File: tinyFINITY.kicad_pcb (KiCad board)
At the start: 2 copper layers, 20 x 20 mm, 111 parts, among them U1 MIC5205, U2 RTC6705, U3 ts3a44159, U4 STM32F301K8Ux, U5 TPS62153A-Q1, X1 8MHZ 20pF 30ppm, X2 8MHz, Y1 LF2012-A5R5AA

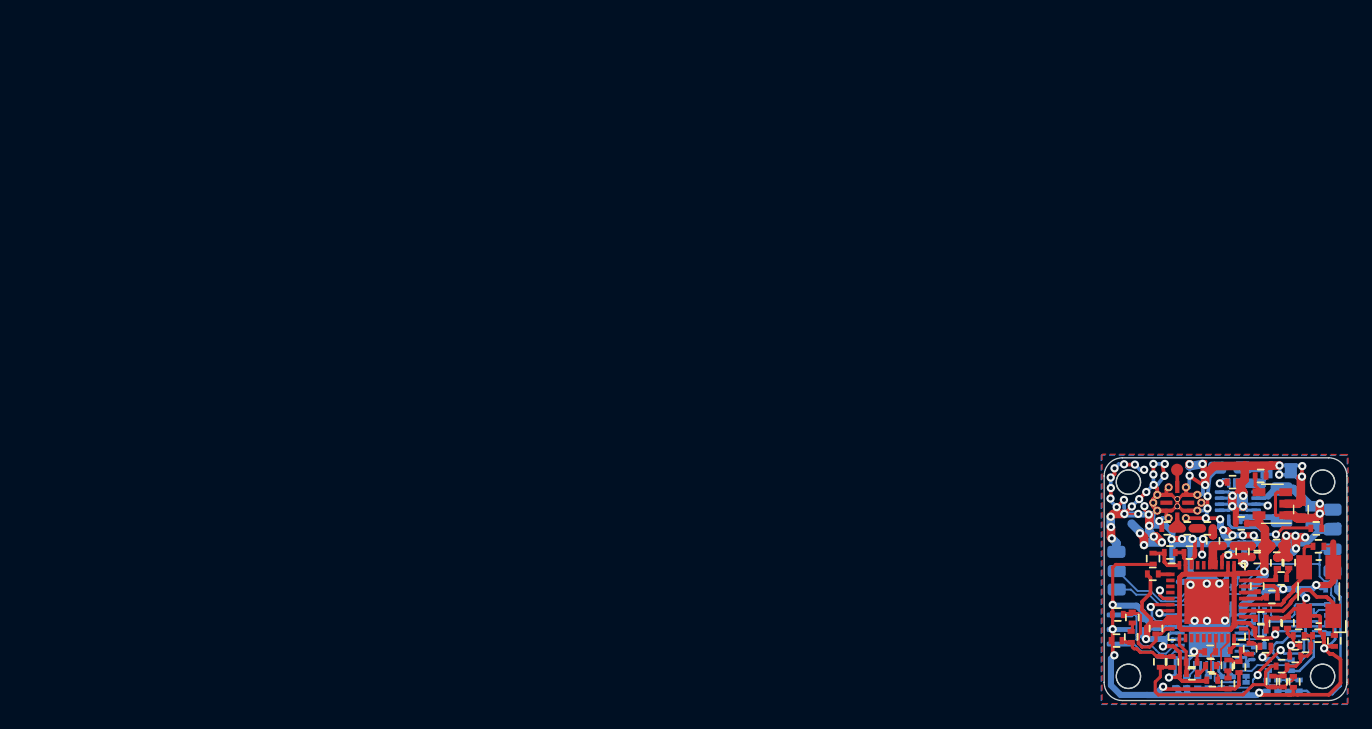
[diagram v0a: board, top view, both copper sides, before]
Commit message: multitabs
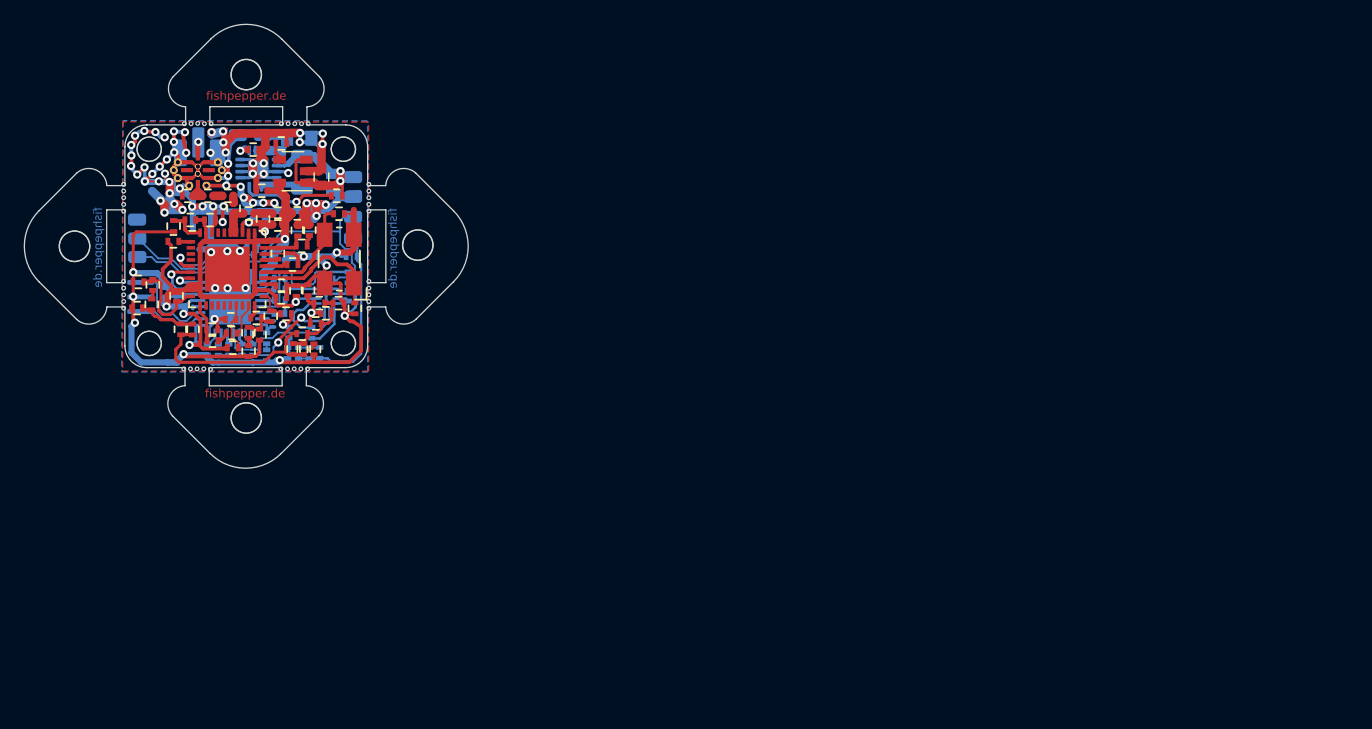
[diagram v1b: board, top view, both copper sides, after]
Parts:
- removed TP12: ANT, custom:smd_1x1_round
- added ANT1: COAX, custom:U.FL-R-SMT-1, B.Cu at (144.6, 97.3)
- added H3: hole, custom:mouting_hole, F.Cu at (153.1, 94.9)
- added H3: hole, custom:mouting_hole, F.Cu at (145.1, 94.9)
- added H3: hole, custom:mouting_hole, F.Cu at (143.9, 115.1)
- added H3: hole, custom:mouting_hole, F.Cu at (145.6, 115.1)
- added H3: hole, custom:mouting_hole, F.Cu at (144.4, 115.1)
- added H3: hole, custom:mouting_hole, F.Cu at (143.3, 115.1)
- added H3: hole, custom:mouting_hole, F.Cu at (145.0, 115.1)
- added H3: hole, custom:mouting_hole, F.Cu at (153.0, 115.1)
- added H3: hole, custom:mouting_hole, F.Cu at (151.3, 115.1)
- added H3: hole, custom:mouting_hole, F.Cu at (152.4, 115.1)
- added H3: hole, custom:mouting_hole, F.Cu at (153.6, 115.1)
- added H3: hole, custom:mouting_hole, F.Cu at (151.4, 94.9)
- added H3: hole, custom:mouting_hole, F.Cu at (151.9, 115.1)
- added H3: hole, custom:mouting_hole, F.Cu at (158.6, 101.5)
- added H3: hole, custom:mouting_hole, F.Cu at (158.6, 99.9)
- added H3: hole, custom:mouting_hole, F.Cu at (158.6, 101.0)
- added H3: hole, custom:mouting_hole, F.Cu at (158.6, 102.1)
- added H3: hole, custom:mouting_hole, F.Cu at (158.6, 100.5)
- added H3: hole, custom:mouting_hole, F.Cu at (158.6, 108.5)
- added H3: hole, custom:mouting_hole, F.Cu at (158.6, 110.1)
- added H3: hole, custom:mouting_hole, F.Cu at (158.6, 109.0)
- added H3: hole, custom:mouting_hole, F.Cu at (158.6, 107.9)
- added H3: hole, custom:mouting_hole, F.Cu at (152.5, 94.9)
- added H3: hole, custom:mouting_hole, F.Cu at (158.6, 109.5)
- added H3: hole, custom:mouting_hole, F.Cu at (138.4, 100.5)
- added H3: hole, custom:mouting_hole, F.Cu at (138.4, 102.1)
- added H3: hole, custom:mouting_hole, F.Cu at (138.4, 101.0)
- added H3: hole, custom:mouting_hole, F.Cu at (138.4, 99.9)
- added H3: hole, custom:mouting_hole, F.Cu at (138.4, 101.5)
- added H3: hole, custom:mouting_hole, F.Cu at (138.4, 109.5)
- added H3: hole, custom:mouting_hole, F.Cu at (138.4, 107.9)
- added H3: hole, custom:mouting_hole, F.Cu at (138.4, 109.0)
- added H3: hole, custom:mouting_hole, F.Cu at (138.4, 110.1)
- added H3: hole, custom:mouting_hole, F.Cu at (153.6, 94.9)
- added H3: hole, custom:mouting_hole, F.Cu at (138.4, 108.5)
- added H3: hole, custom:mouting_hole, F.Cu at (151.9, 94.9)
- added H3: hole, custom:mouting_hole, F.Cu at (143.9, 94.9)
- added H3: hole, custom:mouting_hole, F.Cu at (145.6, 94.9)
- added H3: hole, custom:mouting_hole, F.Cu at (144.5, 94.9)
- added H3: hole, custom:mouting_hole, F.Cu at (143.4, 94.9)
- added H4: hole, custom:mouting_hole, F.Cu at (134.3, 105.0)
- added H4: hole, custom:mouting_hole, F.Cu at (148.5, 90.8)
- added H4: hole, custom:mouting_hole, F.Cu at (162.6, 104.9)
- added H4: hole, custom:mouting_hole, F.Cu at (148.5, 119.2)
- moved H2 87.9 mm to (140.5, 97.0)
- moved C12 85.2 mm to (151.4, 109.2)
- moved C2 85.2 mm to (149.8, 100.4)
- moved C20 85.2 mm to (156.1, 102.3)
- moved C21 85.2 mm to (152.8, 113.8)
- moved C23 85.2 mm to (152.8, 103.7)
- moved C24 85.2 mm to (157.2, 105.8)
- moved C32 85.2 mm to (144.1, 111.9)
- moved C4 85.2 mm to (142.5, 103.3)
- moved C44 85.2 mm to (149.1, 97.0)
- moved D1 85.2 mm to (150.2, 114.0)
- moved R1 85.2 mm to (143.9, 102.8)
- moved R10 85.2 mm to (151.1, 105.6)
- moved R12 85.2 mm to (153.1, 105.0)
- moved R2 85.2 mm to (145.7, 112.8)
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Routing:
- net GND: track 321.4 -> 298.6 mm, vias 79 -> 76
- net Net-(ANT1-PadSIG): track 1.50 -> 1.18 mm, vias 0 -> 1
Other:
- board size 20 x 20 mm -> 36.6 x 36.6 mm
- board text added: "rev 0.3 08/17"
- board text removed: "rev 0.2 08/17"
